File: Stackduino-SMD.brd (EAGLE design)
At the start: 62.5 x 75 mm, 48 parts

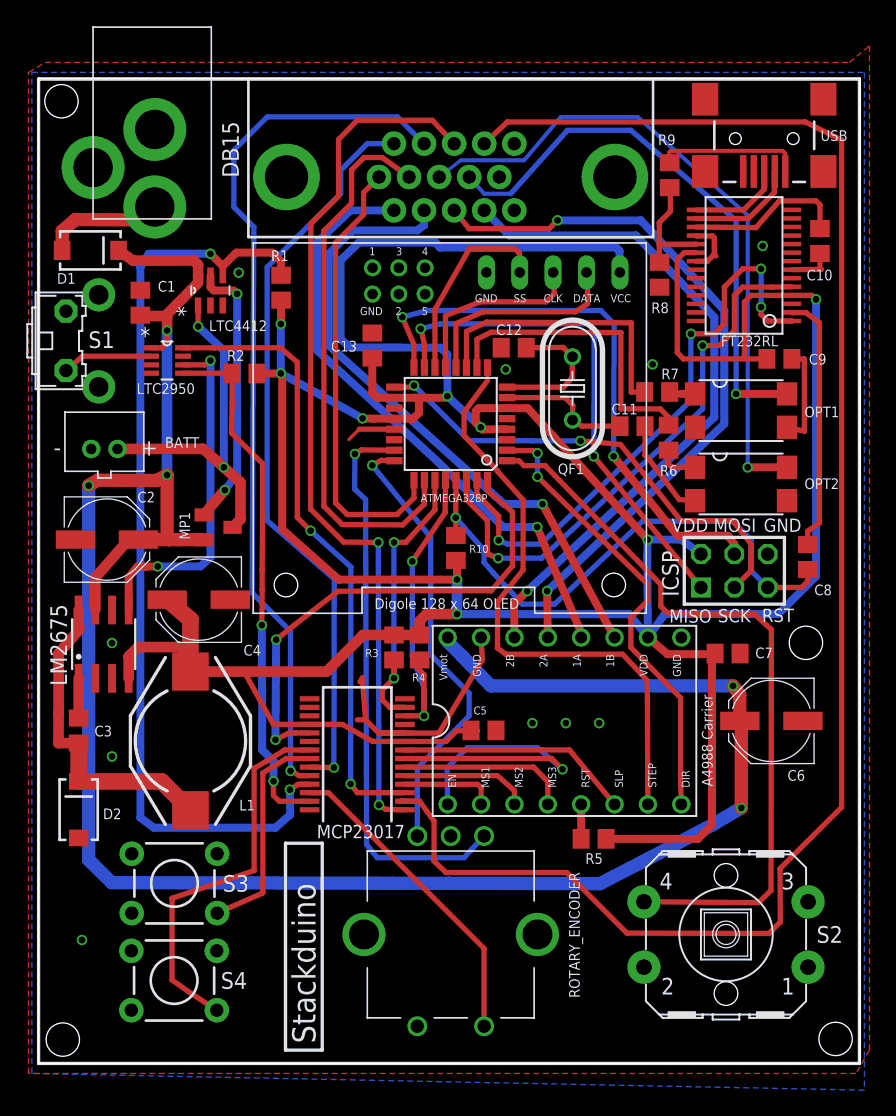
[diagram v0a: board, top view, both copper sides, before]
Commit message: latest progress
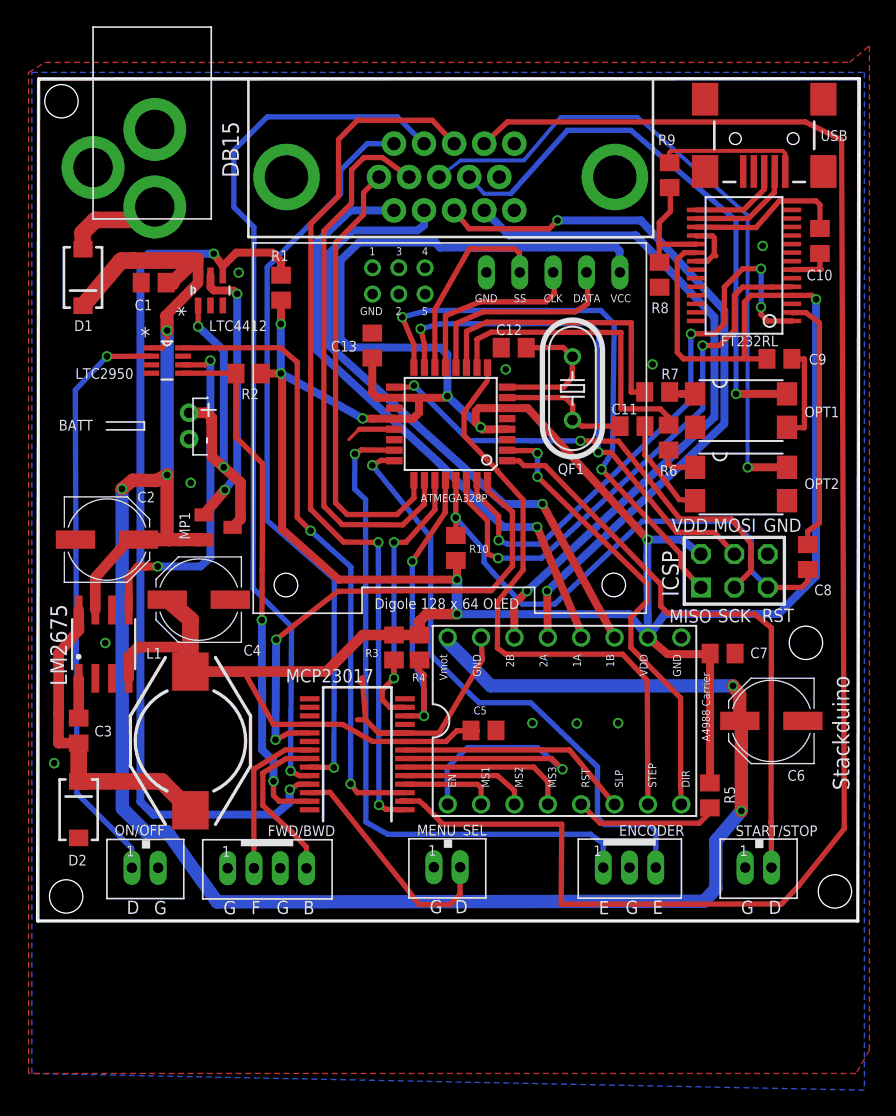
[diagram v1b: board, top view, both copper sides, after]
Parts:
- removed ROTARY_ENCODER: ROTARTY_ENCODER, SparkFun-Electromechanical:ROTARY_ENC_PLAIN
- removed S1: (no value), adafruit:B3F-31XX
- removed S2: (no value), adafruit:B3F-40XX-ROUND
- removed S3: Forward, SparkFun-Electromechanical:TACTILE-PTH
- removed S4: Backward, SparkFun-Electromechanical:TACTILE-PTH
- added ENCODER: JST-PH_3-PIN_HEADER, SRG:JST_B3B-PH_HEADER
- added FWD/BWD: JST-PH_4-PIN_HEADER, SRG:JST_B4B-PH_HEADER
- added MENU_SEL, ON/OFF, START/STOP: JST-PH_2-PIN_HEADER, SRG:JST_B2B-PH_HEADER
- BATT: device adafruit:JST-PH-2-THM -> adafruit:JST-PH-2-THM-RA
- moved R5 9.45 mm to (50.3, 27.5), turned to 90 degrees
- moved BATT 6.69 mm to (10.7, 55.6), turned to 90 degrees
- moved D1 2.13 mm to (2.62, 66.9), turned to 270 degrees
- moved C1 1.83 mm to (8.00, 66.5), turned to 180 degrees
- moved C7 0.38 mm to (51.3, 38.3)
- moved R2 0.30 mm to (15.2, 59.6)
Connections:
- net N$15 renamed XTAL2
- net N$16 renamed XTAL1
- net N$31 renamed PD6
- net N$32 renamed PD7
- removed net N$20: ATMEGA328P.23, ROTARY_ENCODER.A
- removed net N$21: ATMEGA328P.24, ROTARY_ENCODER.B
- new net PC0: ATMEGA328P.23, ENCODER.P1
- new net PC1: ATMEGA328P.24, ENCODER.P3
- net ENCSWITCH: now also MENU_SEL.P2; no longer ROTARY_ENCODER.SW-
- net GND: now also ENCODER.P2, FWD/BWD.P1, FWD/BWD.P3, MENU_SEL.P1, ON/OFF.P2, START/STOP.P1; no longer ROTARY_ENCODER.C, ROTARY_ENCODER.SW+, S1.1, S2.2, S3.2, S4.2
- net MISO: now also ATMEGA328P.16; no longer ATMEGA328P.15
- net MOSI: now also ATMEGA328P.15; no longer ATMEGA328P.16
- net N$28: now also START/STOP.P2; no longer S2.4
- net N$33: now also FWD/BWD.P2; no longer S4.4
- net N$35: now also FWD/BWD.P4; no longer S3.4
- net N$8: now also ON/OFF.P1; no longer S1.2
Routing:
- net PC0: track 0.00 -> 51.8 mm, vias 0 -> 1
- net PC1: track 0.00 -> 45.4 mm, vias 0 -> 1
- net N$20: track 43.3 -> 0.00 mm, vias 1 -> 0
- net N$8: track 6.88 -> 45.0 mm, vias 0 -> 1
- net N$21: track 34.4 -> 0.00 mm, vias 1 -> 0
- net N$33: track 29.3 -> 12.2 mm
- net VCC: track 304.0 -> 291.8 mm
- net N$28: track 56.9 -> 45.1 mm
- net N$2: track 2.63 -> 11.4 mm
- net ENCSWITCH: track 24.1 -> 18.0 mm
- net MISO: track 38.9 -> 43.9 mm
- net N$35: track 16.8 -> 12.5 mm
- net MOSI: track 43.9 -> 39.9 mm
- net V+: track 166.9 -> 169.9 mm
- net VDD: track 27.2 -> 24.6 mm
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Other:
- board size 62.5 x 75 mm -> 62.7 x 64.1 mm
- board text added: "B"
- board text added: "D"
- board text added: "E"
- board text added: "F"
- board text added: "G"

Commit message: Latest progress
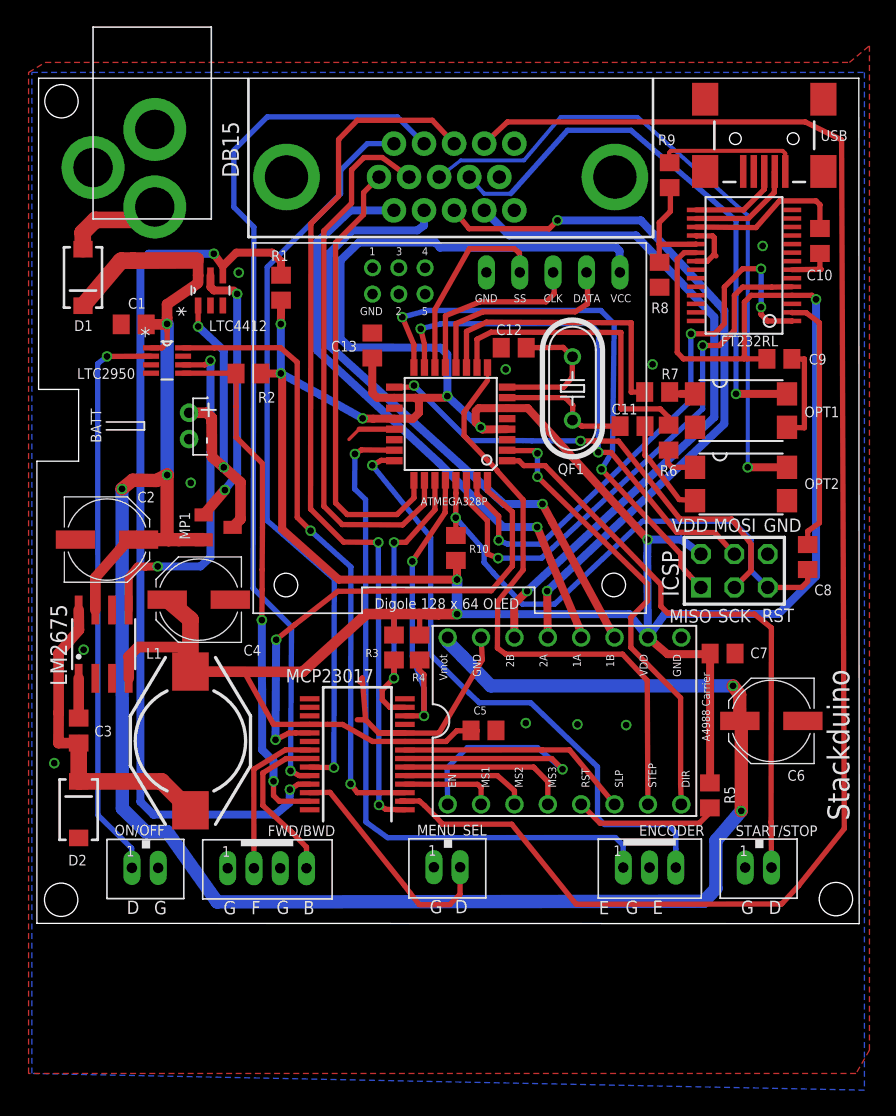
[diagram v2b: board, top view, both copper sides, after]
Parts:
- moved C1 3.52 mm to (6.48, 63.4)
- moved ENCODER 1.52 mm to (45.8, 22.1)
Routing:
- net VCC: track 291.8 -> 295.2 mm
- net DIG2: track 124.3 -> 121.1 mm
- net PC0: track 51.8 -> 53.4 mm
- net PC1: track 45.4 -> 46.9 mm
- net N$8: track 45.0 -> 43.7 mm
- net V+: track 169.9 -> 169.2 mm
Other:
- board size 62.7 x 64.1 mm -> 62.6 x 64.4 mm
